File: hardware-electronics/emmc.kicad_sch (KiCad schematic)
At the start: 44 parts, among them U2 EMMC16G-MW28-01E10, U4 24AA04T-I_OT, U8 USB2244-AEZG-06, Y2 ECS-240-10-47-CKM-TR

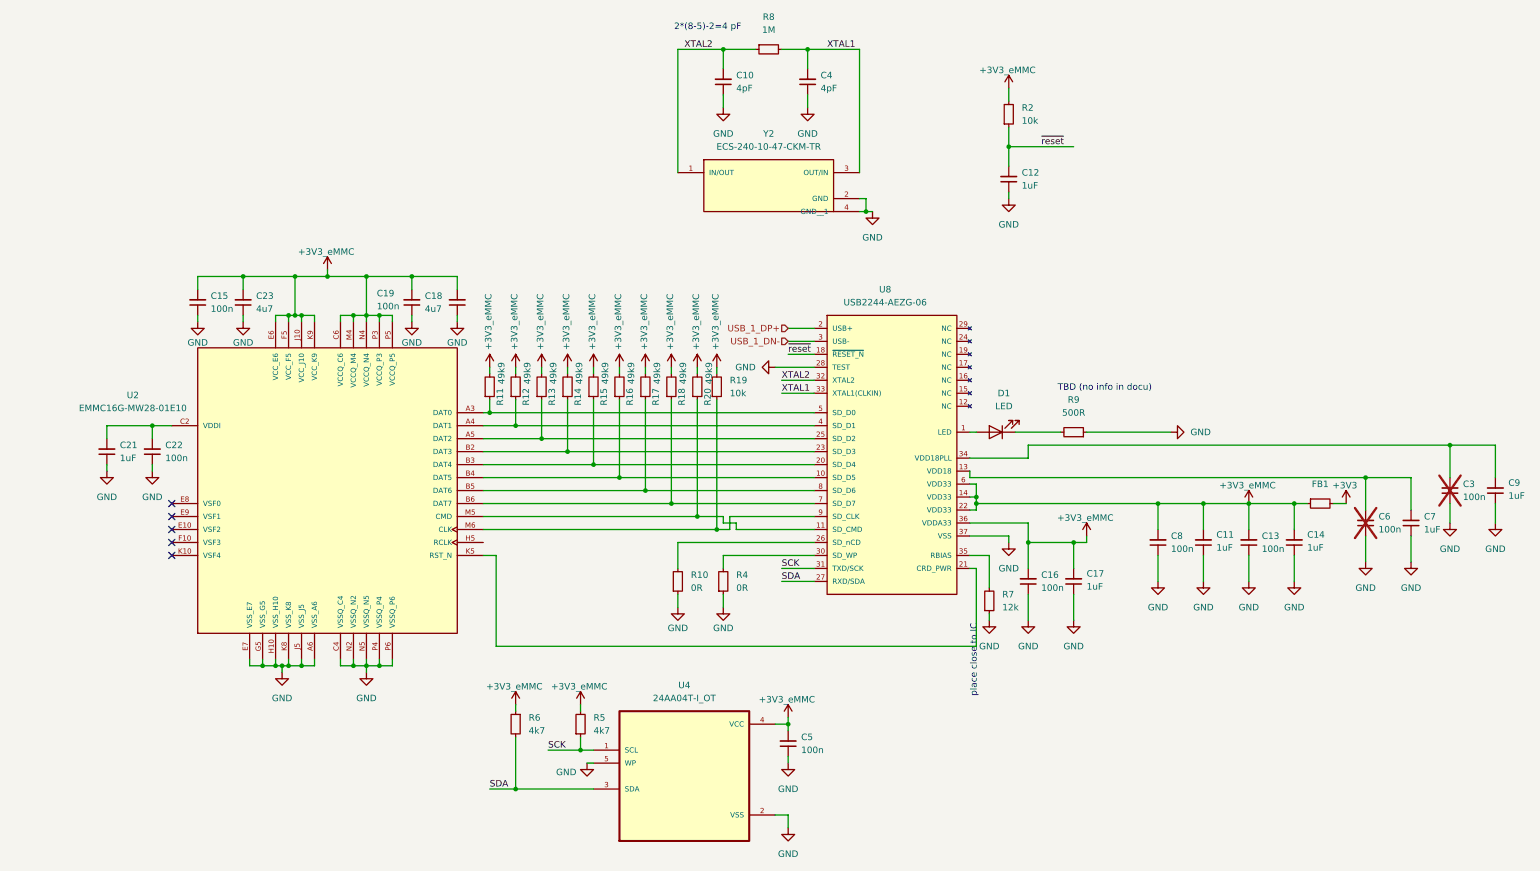
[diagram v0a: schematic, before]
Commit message: SCH cosmetic changes
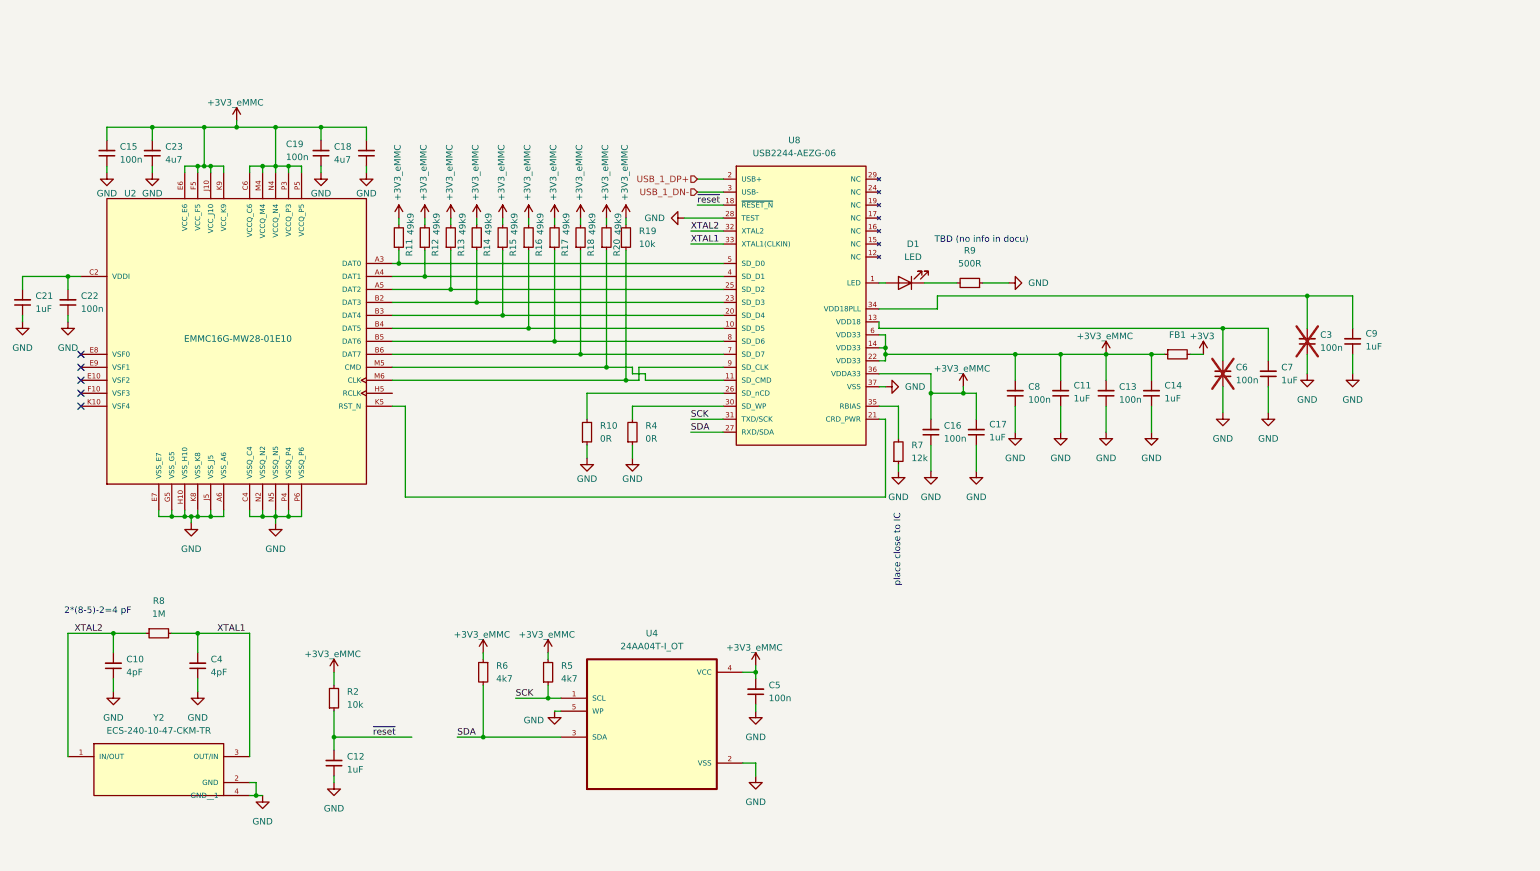
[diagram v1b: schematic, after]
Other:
- moved on the sheet: C10, C11, C12, C13, C14, C15, C16, C17, C18, C19, C21, C22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
